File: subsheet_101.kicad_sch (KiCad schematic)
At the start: 21 parts, among them J10 Joy 1, J11 Mouse / Joy 0, J12 Keyboard, U21 MC6850_PHY

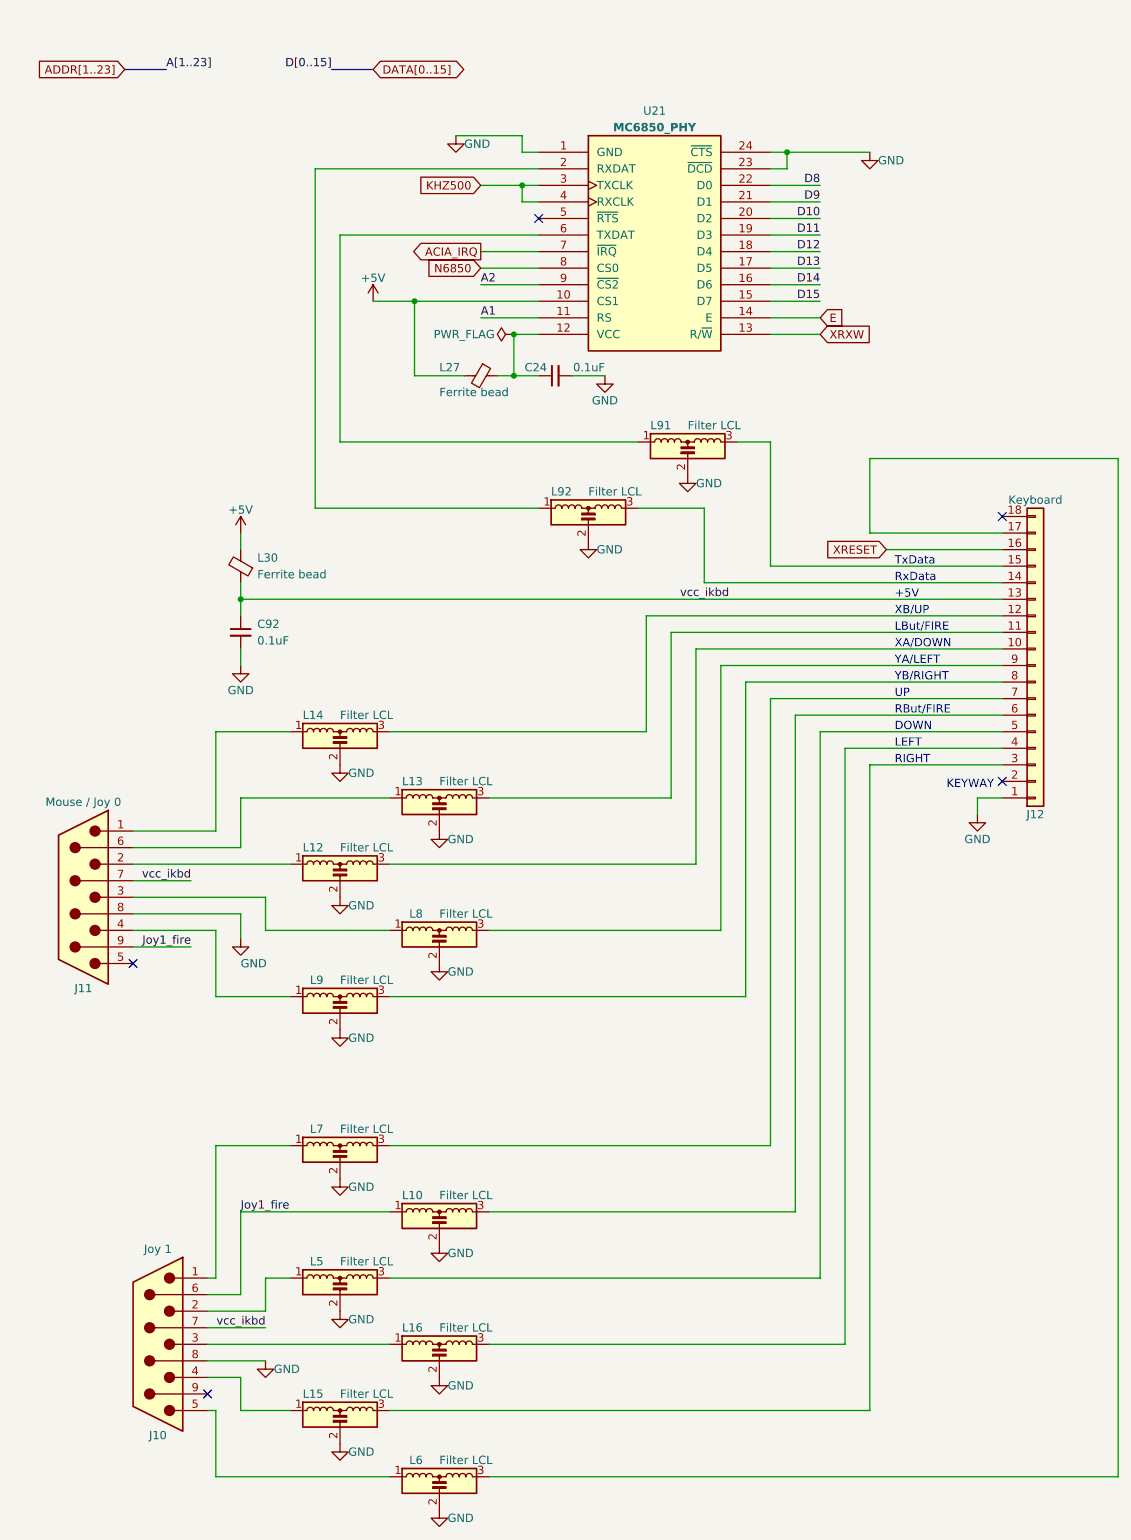
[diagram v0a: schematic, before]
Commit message: fixed power supply of U20 and U21 (ACIAs)
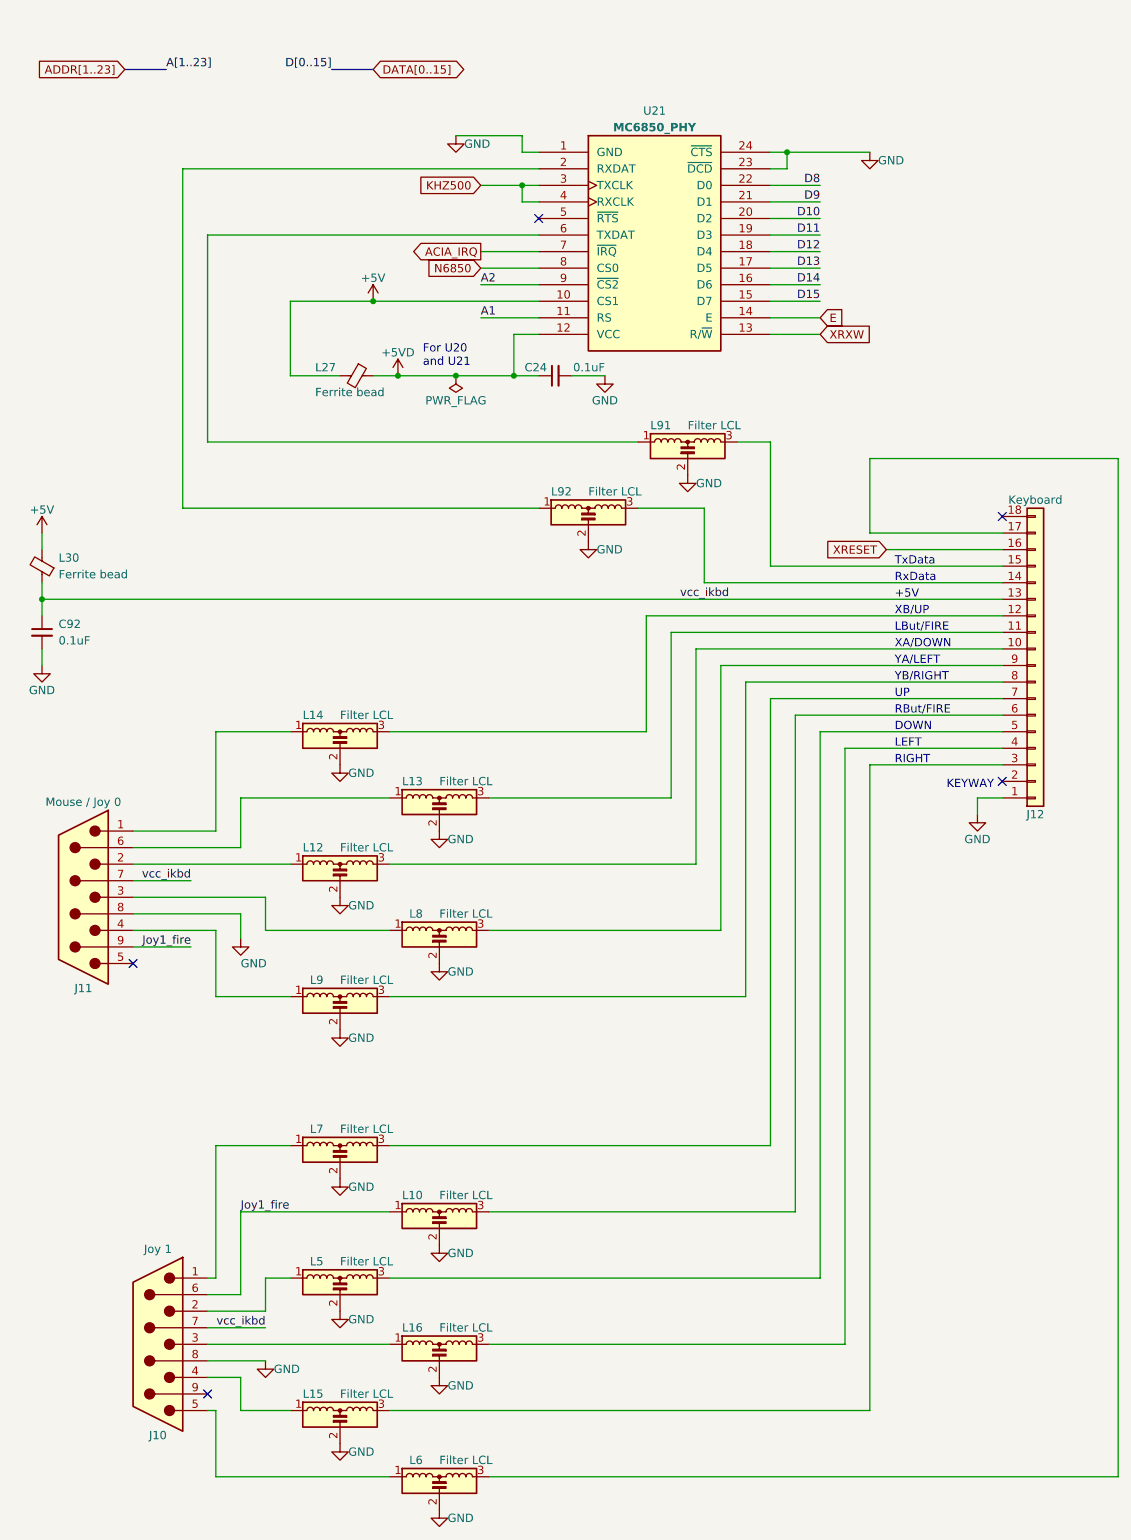
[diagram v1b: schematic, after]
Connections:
- net +5VD: now reaches C24.1, L27.1, U21.12 (VCC)
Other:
- note added: "For U20 and U21"
- moved on the sheet: C92, L27, L30

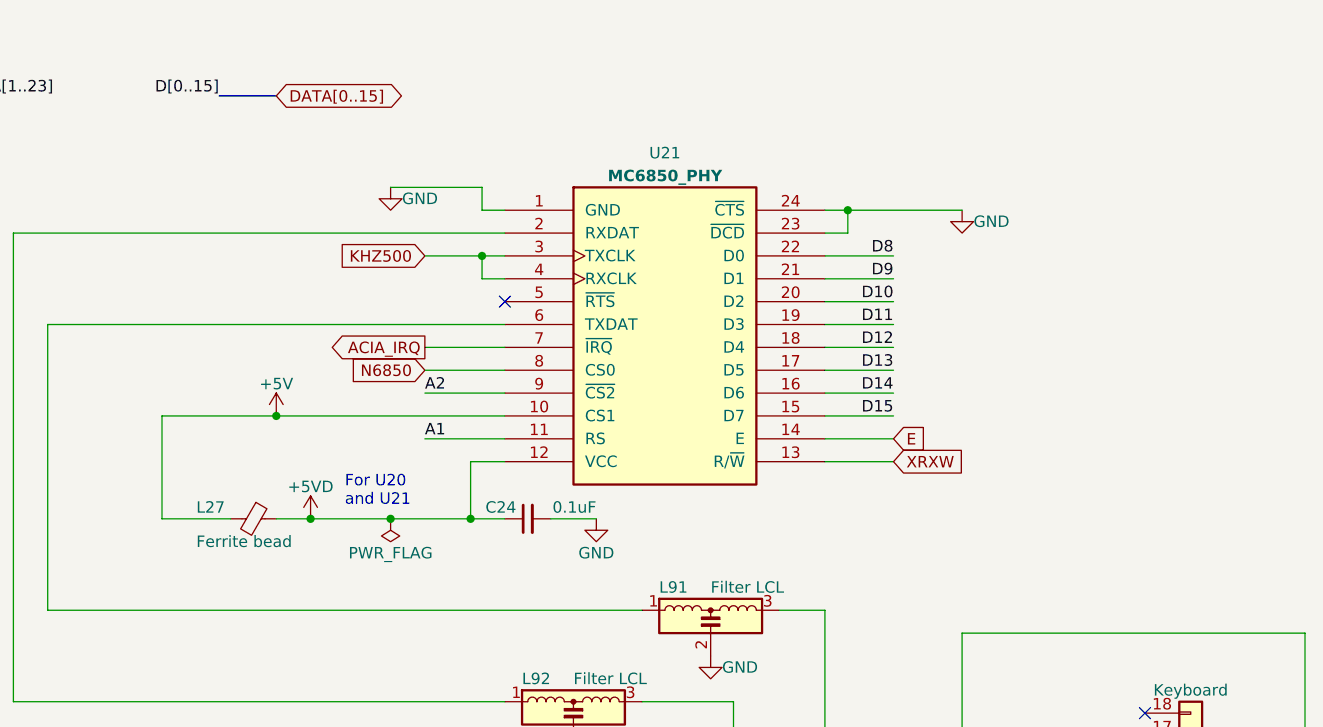
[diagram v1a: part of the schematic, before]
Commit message: fixed U21#10 (ACIA.CS1) -- use same network than U21#12 (ACIA.VCC)
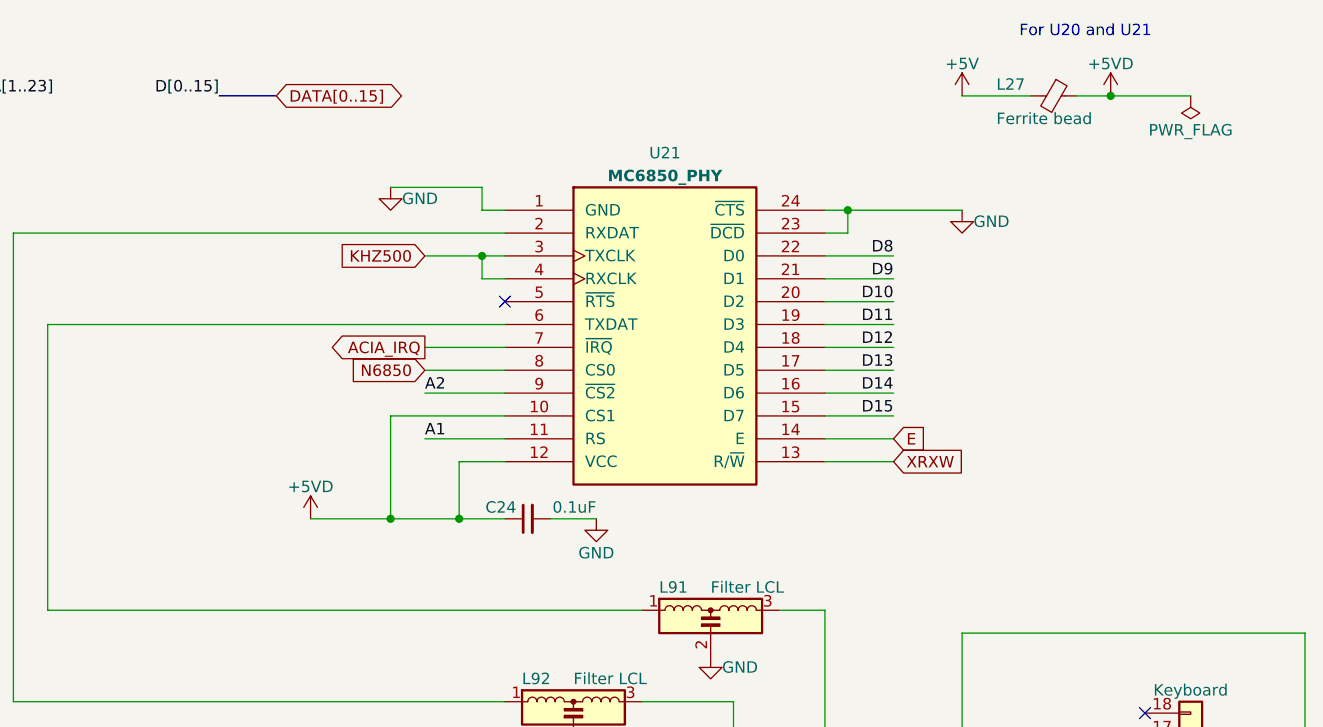
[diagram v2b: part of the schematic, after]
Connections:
- net +5V: no longer U21.10 (CS1)
- net +5VD: now also U21.10 (CS1)
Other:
- moved on the sheet: L27
